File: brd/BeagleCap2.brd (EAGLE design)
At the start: 152.5 x 152 mm, 33 parts, among them IC2 7805TV, J2 DS18B20, J3 Battery, U1 DHT22, X1 Conn BNC : pH, X2 Conn BNC : Dissolved Oxygen, X3 Conn BNC : Conductivity, X4 Conn BNC : ORP

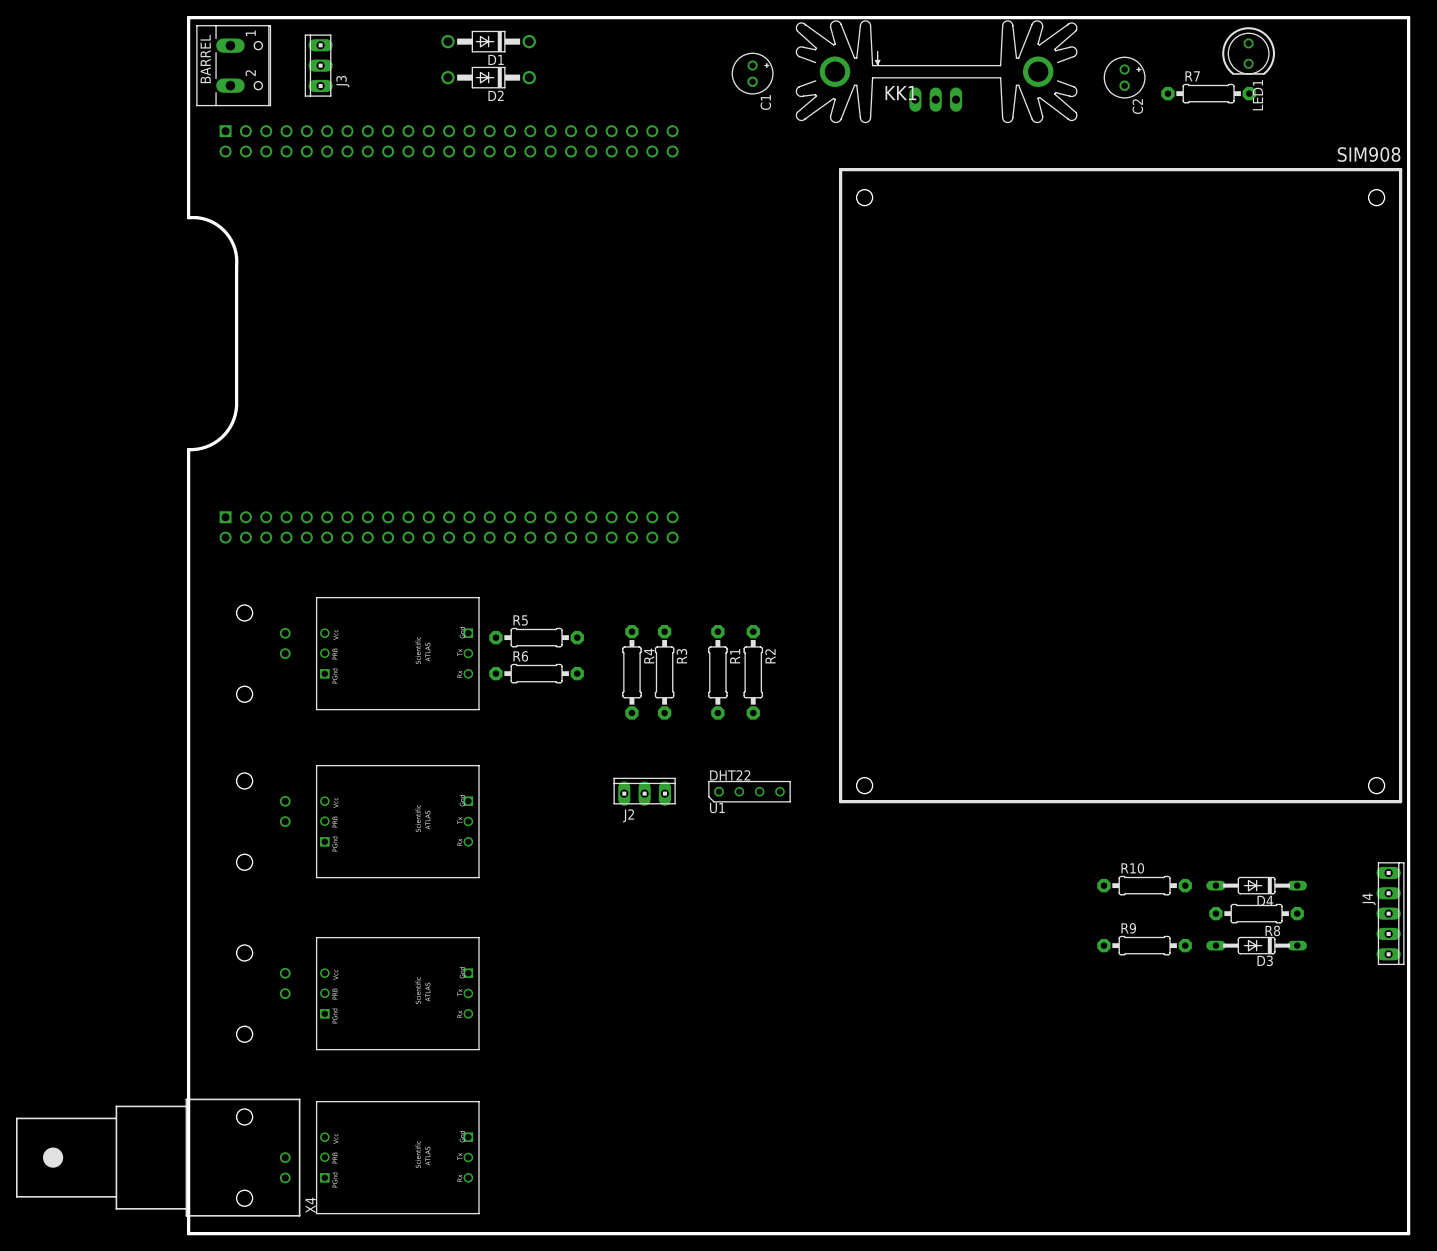
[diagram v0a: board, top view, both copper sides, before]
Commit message: Schematic updated with new PCB
Done by JayMcGee
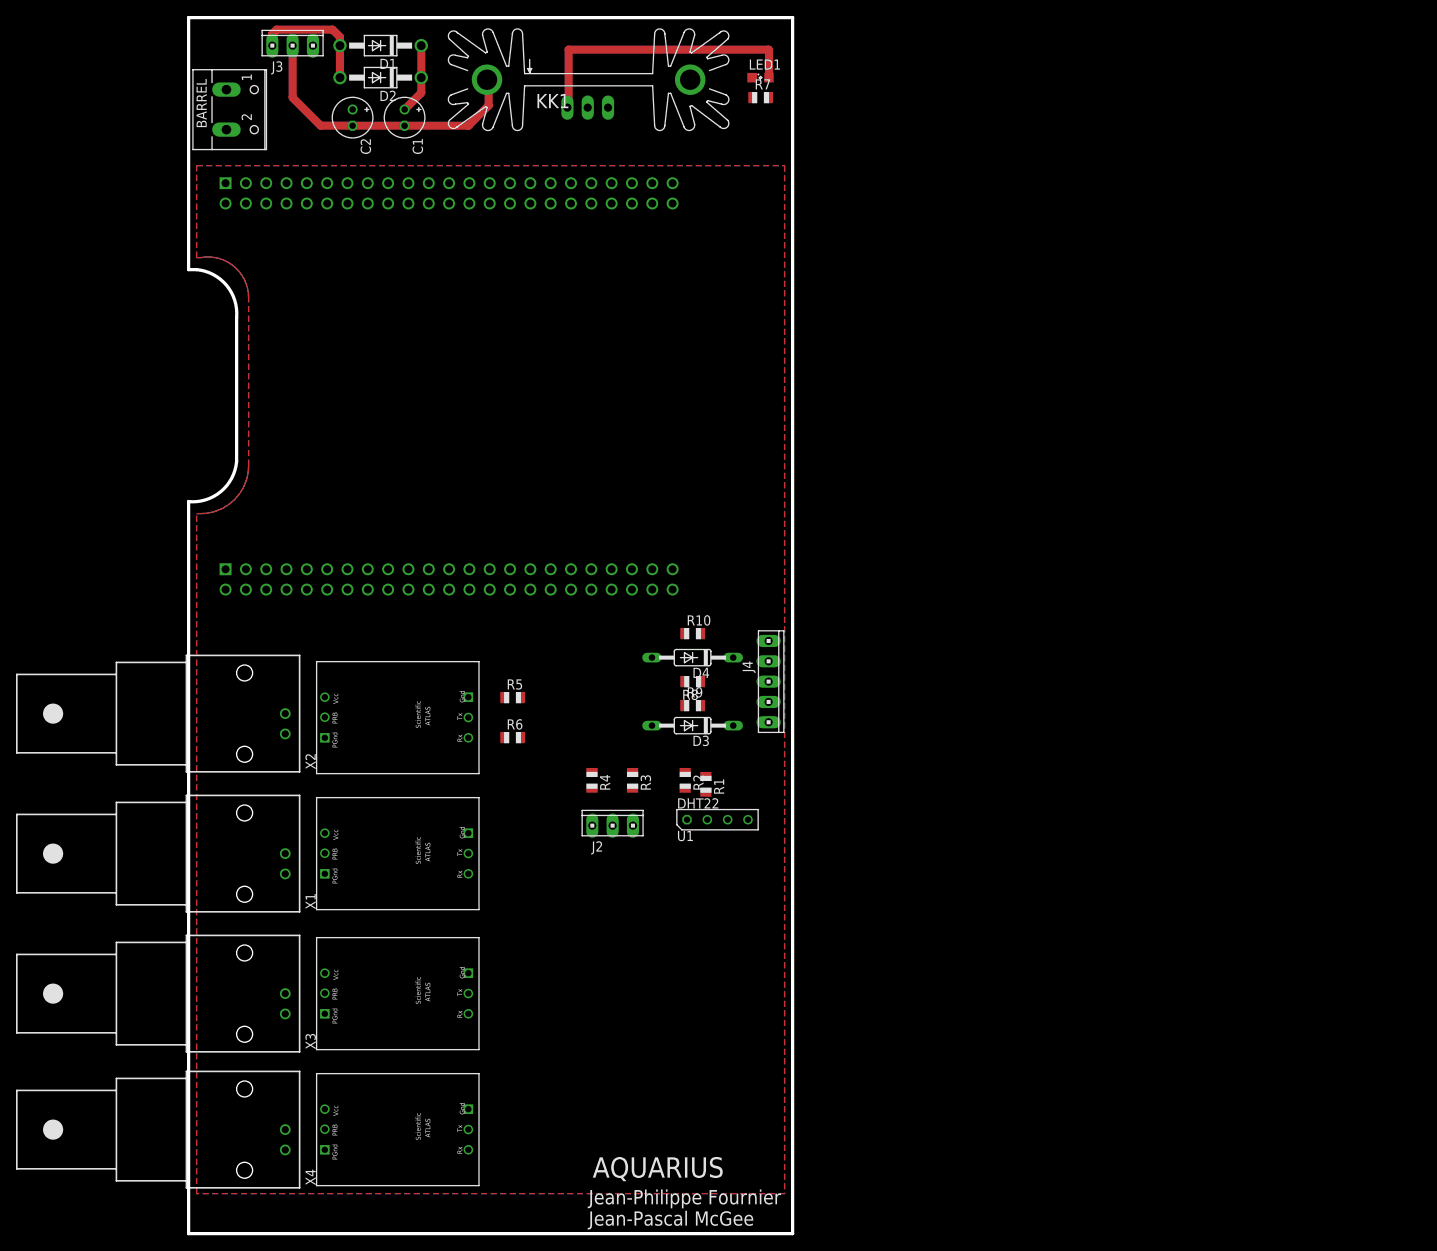
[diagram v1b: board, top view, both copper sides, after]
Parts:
- LED1: device led:LED5MM -> led:SML0805
- R1, R10, R2, R3, R4, R5, R6, R7, R8, R9: device adafruit:0207/10 -> adafruit:R0805
- moved C2 96.6 mm to (-58.5, 76.5)
- moved J4 82.7 mm to (-6.50, 6.00)
- moved R8 76.2 mm to (-16.0, 6.00)
- moved D4 76.0 mm to (-16.0, 9.00)
- moved D3 75.7 mm to (-16.0, 0.50)
- moved R10 64.7 mm to (-16.0, 12.0)
- moved R9 64.0 mm to (-16.0, 3.00)
- moved LED1 61.1 mm to (-7.50, 81.5), turned to 0 degrees
- moved R7 56.0 mm to (-7.50, 79.0)
- moved C1 43.8 mm to (-52.0, 76.5)
- moved IC2 43.5 mm to (-29.1, 80.3)
- moved KK1 43.5 mm to (-29.0, 82.0)
- moved R2 16.0 mm to (-16.9, -6.34)
- moved R4 14.4 mm to (-28.6, -6.34)
- moved R1 14.1 mm to (-14.3, -6.84)
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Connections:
- net 3.3V renamed GNDX
- net N$2: now also LED1.C; no longer LED1.K
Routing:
- net GND: track 0.00 -> 36.8 mm
- net 5V: track 0.00 -> 35.8 mm
- net N$1: track 0.00 -> 15.6 mm
- net VIN: track 0.00 -> 8.85 mm
- added copper zone on layer 16, net GND
- added copper zone on layer 1, net GNDX
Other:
- board size 152.5 x 152 mm -> 75.5 x 152 mm
- board text added: "AQUARIUS"
- board text added: "Jean-Philippe Fournier Jean-Pascal McGee"
- board text removed: "SIM908"
